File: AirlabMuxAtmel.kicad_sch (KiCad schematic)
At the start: 2 parts, among them IC1 ATXMEGA128A4U#TQFP44, IC2 80C552

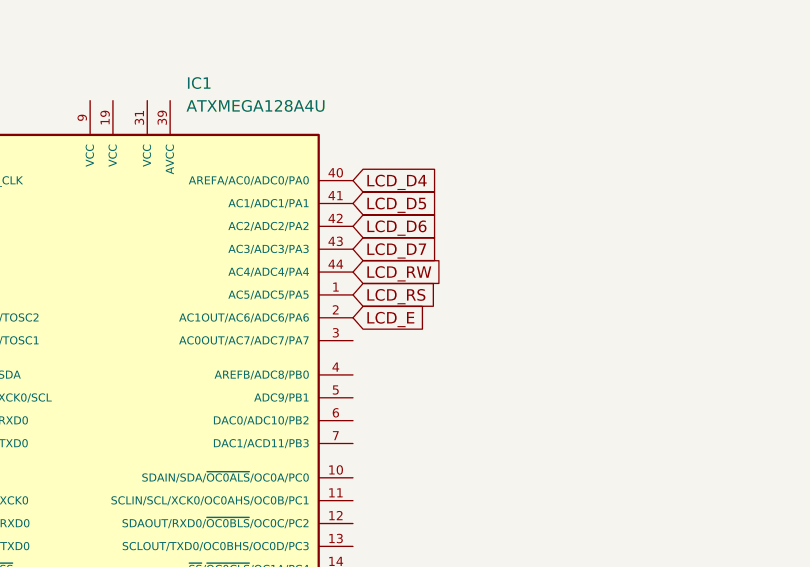
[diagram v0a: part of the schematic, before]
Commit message: ok
ok
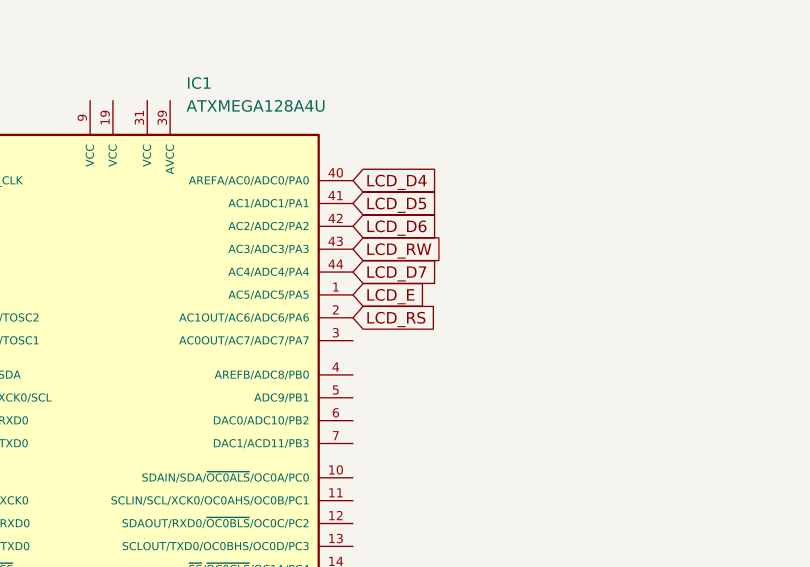
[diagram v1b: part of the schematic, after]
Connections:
- net LCD_D7: now also IC1.44 (AC4/ADC4/PA4); no longer IC1.43 (AC3/ADC3/PA3)
- net LCD_E: now also IC1.1 (AC5/ADC5/PA5); no longer IC1.2 (AC1OUT/AC6/ADC6/PA6)
- net LCD_RS: now also IC1.2 (AC1OUT/AC6/ADC6/PA6); no longer IC1.1 (AC5/ADC5/PA5)
- net LCD_RW: now also IC1.43 (AC3/ADC3/PA3); no longer IC1.44 (AC4/ADC4/PA4)
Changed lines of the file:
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@@
     )
   )
-  (global_label "LCD_RS" (shape input) (at 119.38 67.945 0) (fields_autoplaced)
+  (global_label "LCD_RS" (shape input) (at 119.38 70.485 0) (fields_autoplaced)
     (effects (font (size 1.27 1.27)) (justify left))
-    (property "Intersheet References" "${INTERSHEET_REFS}" (id 0) (at 128.8083 67.8656 0)
+    (property "Intersheet References" "${INTERSHEET_REFS}" (id 0) (at 128.8083 70.4056 0)
       (effects (font (size 1.27 1.27)) (justify left) hide)
     )
@@
     )
   )
-  (global_label "LCD_D7" (shape input) (at 119.38 62.865 0) (fields_autoplaced)
+  (global_label "LCD_D7" (shape input) (at 119.38 65.405 0) (fields_autoplaced)
     (effects (font (size 1.27 1.27)) (justify left))
-    (property "Intersheet References" "${INTERSHEET_REFS}" (id 0) (at 128.8083 62.7856 0)
+    (property "Intersheet References" "${INTERSHEET_REFS}" (id 0) (at 128.8083 65.3256 0)
       (effects (font (size 1.27 1.27)) (justify left) hide)
     )
@@
     )
   )
-  (global_label "LCD_RW" (shape input) (at 119.38 65.405 0) (fields_autoplaced)
+  (global_label "LCD_RW" (shape input) (at 119.38 62.865 0) (fields_autoplaced)
     (effects (font (size 1.27 1.27)) (justify left))
-    (property "Intersheet References" "${INTERSHEET_REFS}" (id 0) (at 129.0502 65.3256 0)
+    (property "Intersheet References" "${INTERSHEET_REFS}" (id 0) (at 129.0502 62.7856 0)
       (effects (font (size 1.27 1.27)) (justify left) hide)
     )
   )
-  (global_label "LCD_E" (shape input) (at 119.38 70.485 0) (fields_autoplaced)
+  (global_label "LCD_E" (shape input) (at 119.38 67.945 0) (fields_autoplaced)
     (effects (font (size 1.27 1.27)) (justify left))
-    (property "Intersheet References" "${INTERSHEET_REFS}" (id 0) (at 127.4779 70.4056 0)
+    (property "Intersheet References" "${INTERSHEET_REFS}" (id 0) (at 127.4779 67.8656 0)
       (effects (font (size 1.27 1.27)) (justify left) hide)
     )

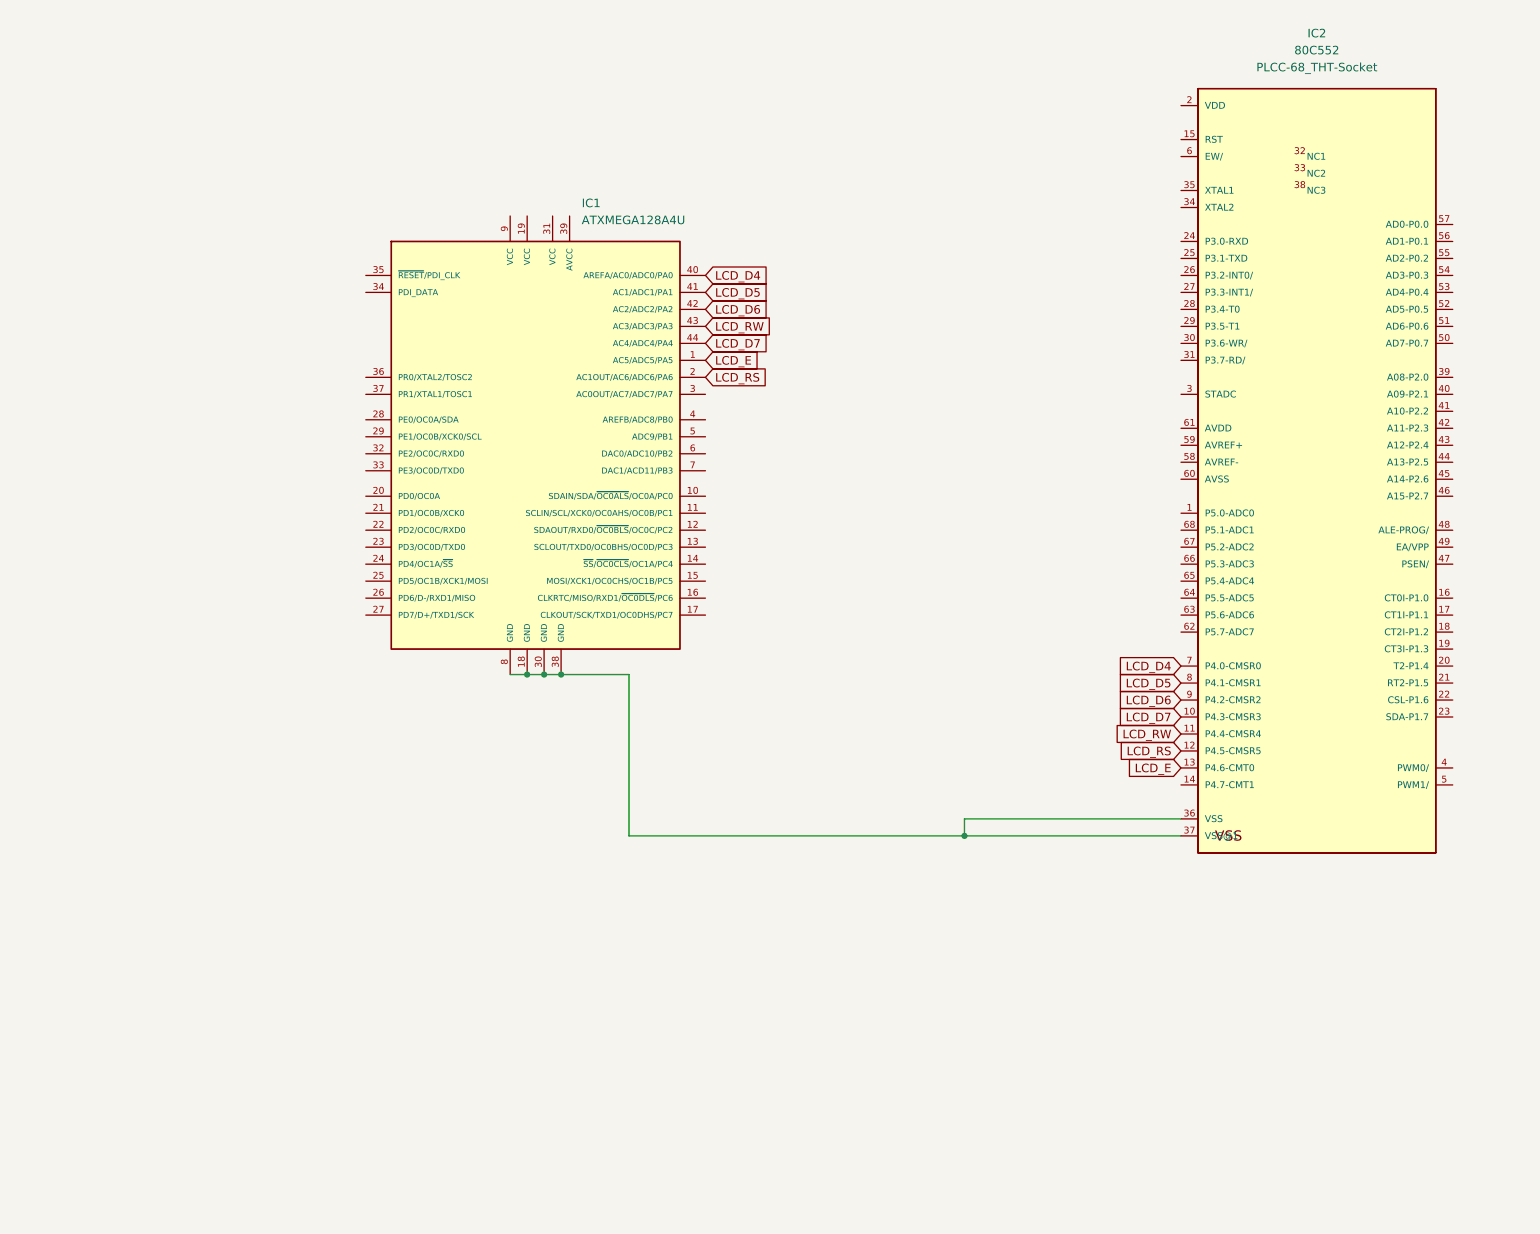
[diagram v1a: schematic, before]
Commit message: oke
oke
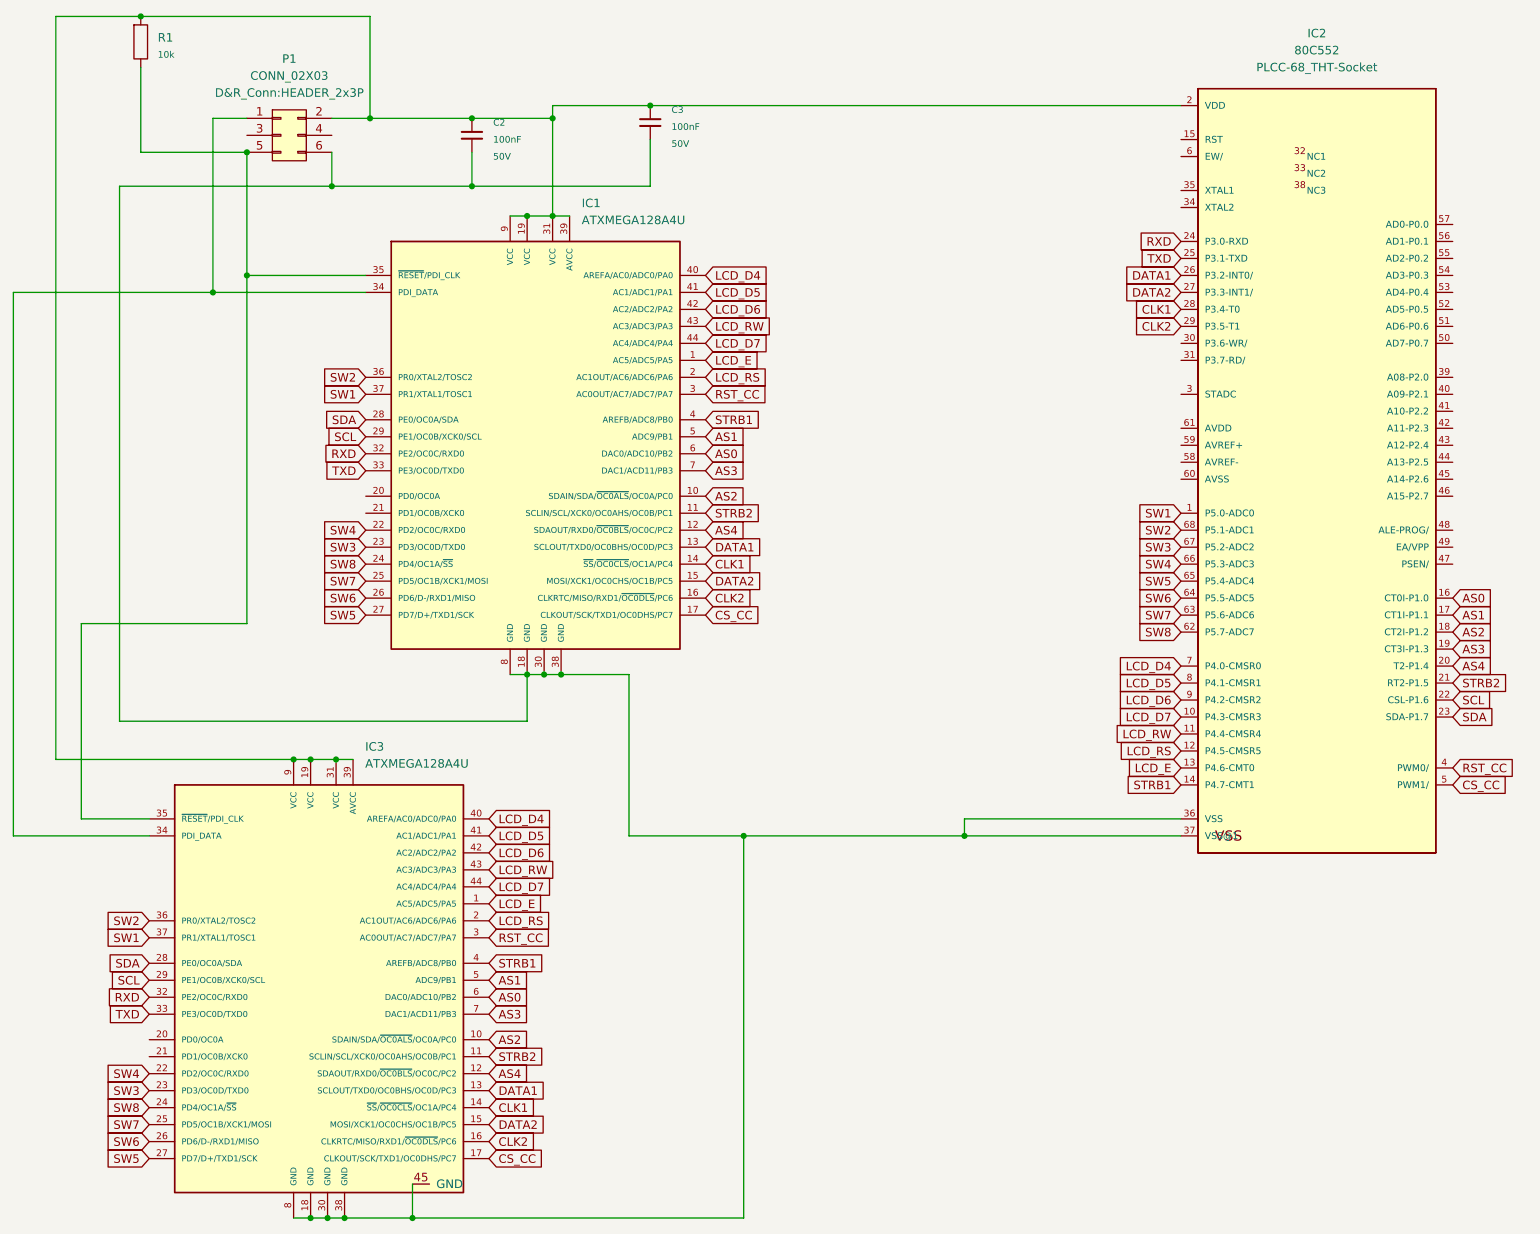
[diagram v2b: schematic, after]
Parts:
- added C2, C3: 100N-X7R_50V#0603-D&R_Passive, D&R_Passive:C_0603, symbol D&R_other:100N-X7R_50V#0603-D&R_Passive
- added IC3: ATXMEGA128A4U#TQFP44, Package_qfn:QFN50P700X700X100-45N, symbol D&R_IC:ATXMEGA128A4U#TQFP44
- added P1: CONN_02X03, D&R_Conn:HEADER_2x3P, symbol D&R_Conn:CONN_02X03
- added R1: 0R#0603, D&R_Passive:R_0603, symbol D&R_Passive:0R#0603
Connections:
- net LCD_D4: now also IC3.40 (AREFA/AC0/ADC0/PA0)
- net LCD_D5: now also IC3.41 (AC1/ADC1/PA1)
- net LCD_D6: now also IC3.42 (AC2/ADC2/PA2)
- net LCD_D7: now also IC3.44 (AC4/ADC4/PA4)
- net LCD_E: now also IC3.1 (AC5/ADC5/PA5)
- net LCD_RS: now also IC3.2 (AC1OUT/AC6/ADC6/PA6)
- net LCD_RW: now also IC3.43 (AC3/ADC3/PA3)
- net AS2: now reaches IC1.10 (SDAIN/SDA/~{OC0ALS}/OC0A/PC0)
- net AS2: now also IC2.18 (CT2I-P1.2), IC3.10 (SDAIN/SDA/~{OC0ALS}/OC0A/PC0)
- net STRB2: now reaches IC1.11 (SCLIN/SCL/XCK0/OC0AHS/OC0B/PC1)
- net STRB2: now also IC2.21 (RT2-P1.5), IC3.11 (SCLIN/SCL/XCK0/OC0AHS/OC0B/PC1)
- net AS4: now reaches IC1.12 (SDAOUT/RXD0/~{OC0BLS}/OC0C/PC2)
- net AS4: now also IC2.20 (T2-P1.4), IC3.12 (SDAOUT/RXD0/~{OC0BLS}/OC0C/PC2)
- net DATA1: now reaches IC1.13 (SCLOUT/TXD0/OC0BHS/OC0D/PC3)
- net DATA1: now also IC2.26 (P3.2-INT0/), IC3.13 (SCLOUT/TXD0/OC0BHS/OC0D/PC3)
- net CLK1: now reaches IC1.14 (~{SS}/~{OC0CLS}/OC1A/PC4)
- net CLK1: now also IC2.28 (P3.4-T0), IC3.14 (~{SS}/~{OC0CLS}/OC1A/PC4)
- net DATA2: now reaches IC1.15 (MOSI/XCK1/OC0CHS/OC1B/PC5)
- net DATA2: now also IC2.27 (P3.3-INT1/), IC3.15 (MOSI/XCK1/OC0CHS/OC1B/PC5)
- net CLK2: now reaches IC1.16 (CLKRTC/MISO/RXD1/~{OC0DLS}/PC6)
- net CLK2: now also IC2.29 (P3.5-T1), IC3.16 (CLKRTC/MISO/RXD1/~{OC0DLS}/PC6)
- net CS_CC: now reaches IC1.17 (CLKOUT/SCK/TXD1/OC0DHS/PC7)
- net CS_CC: now also IC2.5 (PWM1/), IC3.17 (CLKOUT/SCK/TXD1/OC0DHS/PC7)
- net at IC1.18 (GND), IC1.30 (GND), IC1.38 (GND)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: now also C2.2, C3.2, IC3.18 (GND), IC3.30 (GND), IC3.38 (GND), IC3.45 (GND), IC3.8 (GND), P1.6 (P6)
- net at IC1.19 (VCC): now also IC1.31 (VCC), IC1.39 (AVCC), IC1.9 (VCC), IC2.2 (VDD), C2.1, C3.1, IC3.19 (VCC), IC3.31 (VCC), IC3.39 (AVCC), IC3.9 (VCC), P1.2 (P2), R1.1
- net SW4: now reaches IC1.22 (PD2/OC0C/RXD0)
- net SW4: now also IC2.66 (P5.3-ADC3), IC3.22 (PD2/OC0C/RXD0)
- net SW3: now reaches IC1.23 (PD3/OC0D/TXD0)
- net SW3: now also IC2.67 (P5.2-ADC2), IC3.23 (PD3/OC0D/TXD0)
- net SW8: now reaches IC1.24 (PD4/OC1A/~{SS})
- net SW8: now also IC2.62 (P5.7-ADC7), IC3.24 (PD4/OC1A/~{SS})
- net SW7: now reaches IC1.25 (PD5/OC1B/XCK1/MOSI)
- net SW7: now also IC2.63 (P5.6-ADC6), IC3.25 (PD5/OC1B/XCK1/MOSI)
- net SW6: now reaches IC1.26 (PD6/D-/RXD1/MISO)
- net SW6: now also IC2.64 (P5.5-ADC5), IC3.26 (PD6/D-/RXD1/MISO)
- net SW5: now reaches IC1.27 (PD7/D+/TXD1/SCK)
- net SW5: now also IC2.65 (P5.4-ADC4), IC3.27 (PD7/D+/TXD1/SCK)
- net SDA: now reaches IC1.28 (PE0/OC0A/SDA)
- net SDA: now also IC2.23 (SDA-P1.7), IC3.28 (PE0/OC0A/SDA)
- net SCL: now reaches IC1.29 (PE1/OC0B/XCK0/SCL)
- net SCL: now also IC2.22 (CSL-P1.6), IC3.29 (PE1/OC0B/XCK0/SCL)
- net RST_CC: now reaches IC1.3 (AC0OUT/AC7/ADC7/PA7)
- net RST_CC: now also IC2.4 (PWM0/), IC3.3 (AC0OUT/AC7/ADC7/PA7)
- net RXD: now reaches IC1.32 (PE2/OC0C/RXD0)
- net RXD: now also IC2.24 (P3.0-RXD), IC3.32 (PE2/OC0C/RXD0)
- net TXD: now reaches IC1.33 (PE3/OC0D/TXD0)
- net TXD: now also IC2.25 (P3.1-TXD), IC3.33 (PE3/OC0D/TXD0)
- net at IC1.34 (PDI_DATA): now also IC3.34 (PDI_DATA), P1.1 (P1)
- net at IC1.35 (~{RESET}/PDI_CLK): now also IC3.35 (~{RESET}/PDI_CLK), P1.5 (P5), R1.2
- net SW2: now reaches IC1.36 (PR0/XTAL2/TOSC2)
- net SW2: now also IC2.68 (P5.1-ADC1), IC3.36 (PR0/XTAL2/TOSC2)
- net SW1: now reaches IC1.37 (PR1/XTAL1/TOSC1)
- net SW1: now also IC2.1 (P5.0-ADC0), IC3.37 (PR1/XTAL1/TOSC1)
- net STRB1: now reaches IC1.4 (AREFB/ADC8/PB0)
- net STRB1: now also IC2.14 (P4.7-CMT1), IC3.4 (AREFB/ADC8/PB0)
- net AS1: now reaches IC1.5 (ADC9/PB1)
- net AS1: now also IC2.17 (CT1I-P1.1), IC3.5 (ADC9/PB1)
- net AS0: now reaches IC1.6 (DAC0/ADC10/PB2)
- net AS0: now also IC2.16 (CT0I-P1.0), IC3.6 (DAC0/ADC10/PB2)
- net AS3: now reaches IC1.7 (DAC1/ACD11/PB3)
- net AS3: now also IC2.19 (CT3I-P1.3), IC3.7 (DAC1/ACD11/PB3)
